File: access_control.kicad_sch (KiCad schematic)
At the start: 64 parts, among them J1 Conn_01x04_Pin, J10 Screw_Terminal_01x02, J2 Screw_Terminal_01x04, J3 Screw_Terminal_01x04, J4 Screw_Terminal_01x02, J5 Screw_Terminal_01x04, J6 Screw_Terminal_01x04, J7 Screw_Terminal_01x02, J8 Screw_Terminal_01x02, J9 Screw_Terminal_01x02, Q1 NMOS, Q2 NMOS, Q3 NMOS, Q4 NMOS, SW1 Reset button, U1 STM32F446RETx, U2 DS3231M, U3 MAX3232ESE, U4 MAX3232ESE, U5 BA033CC0T, Y1 16MHz

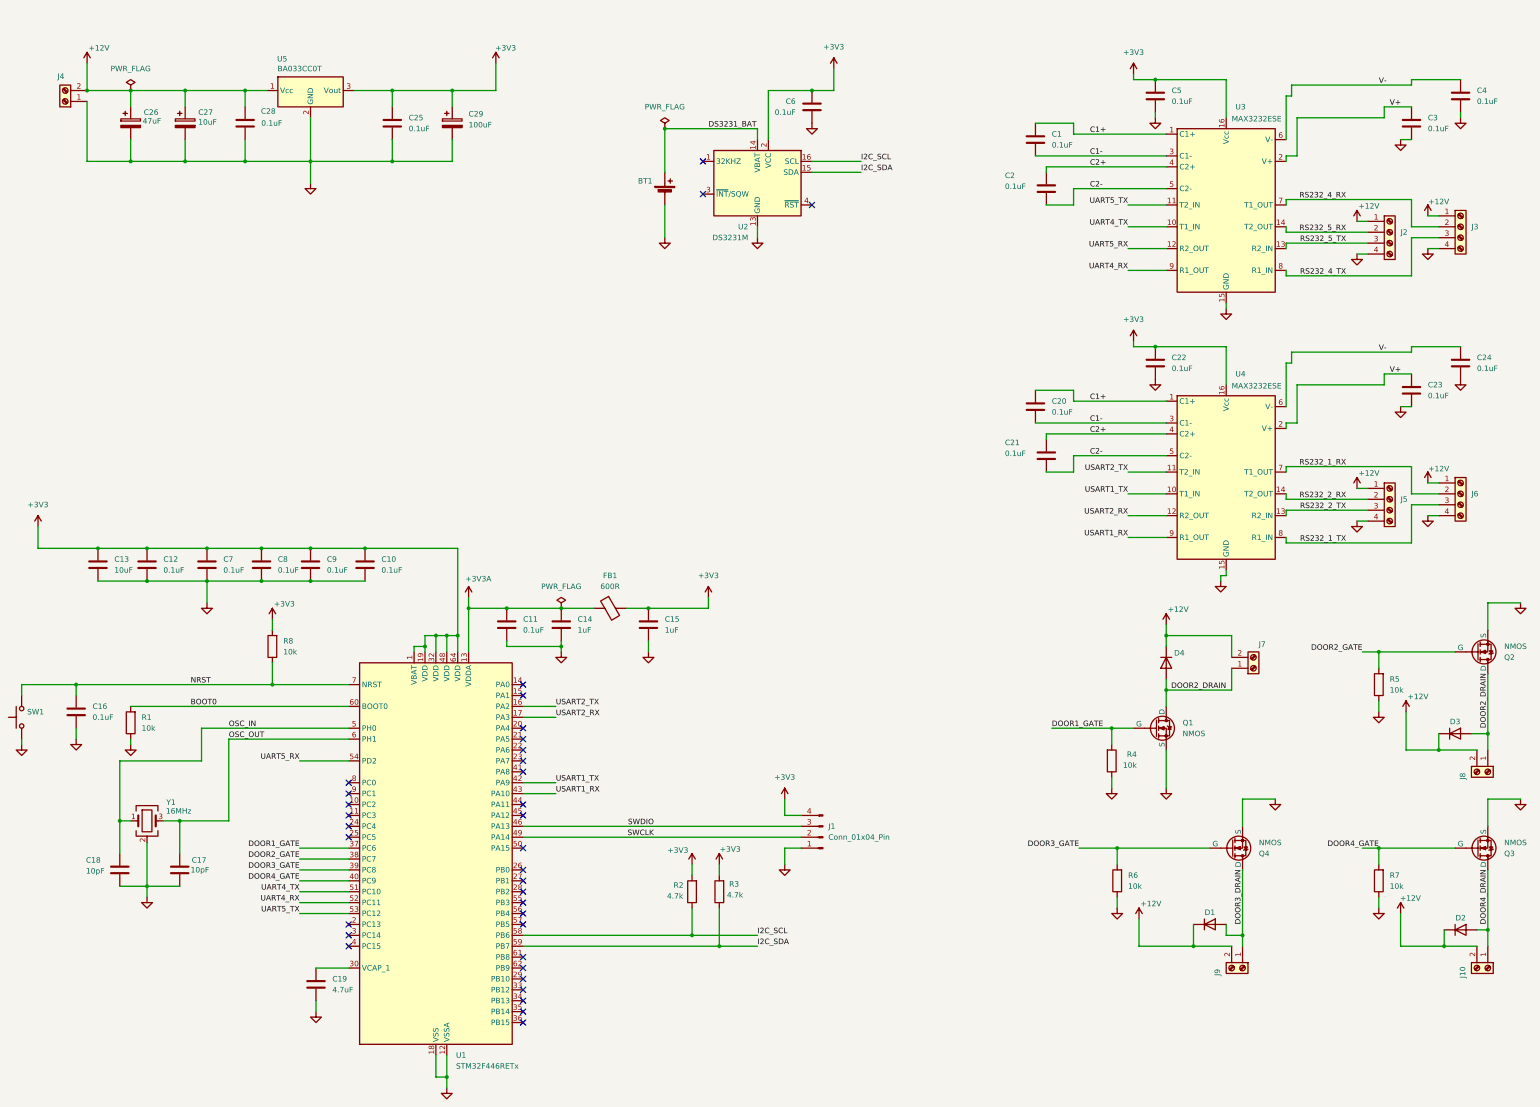
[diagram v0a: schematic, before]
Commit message: ERC check verified
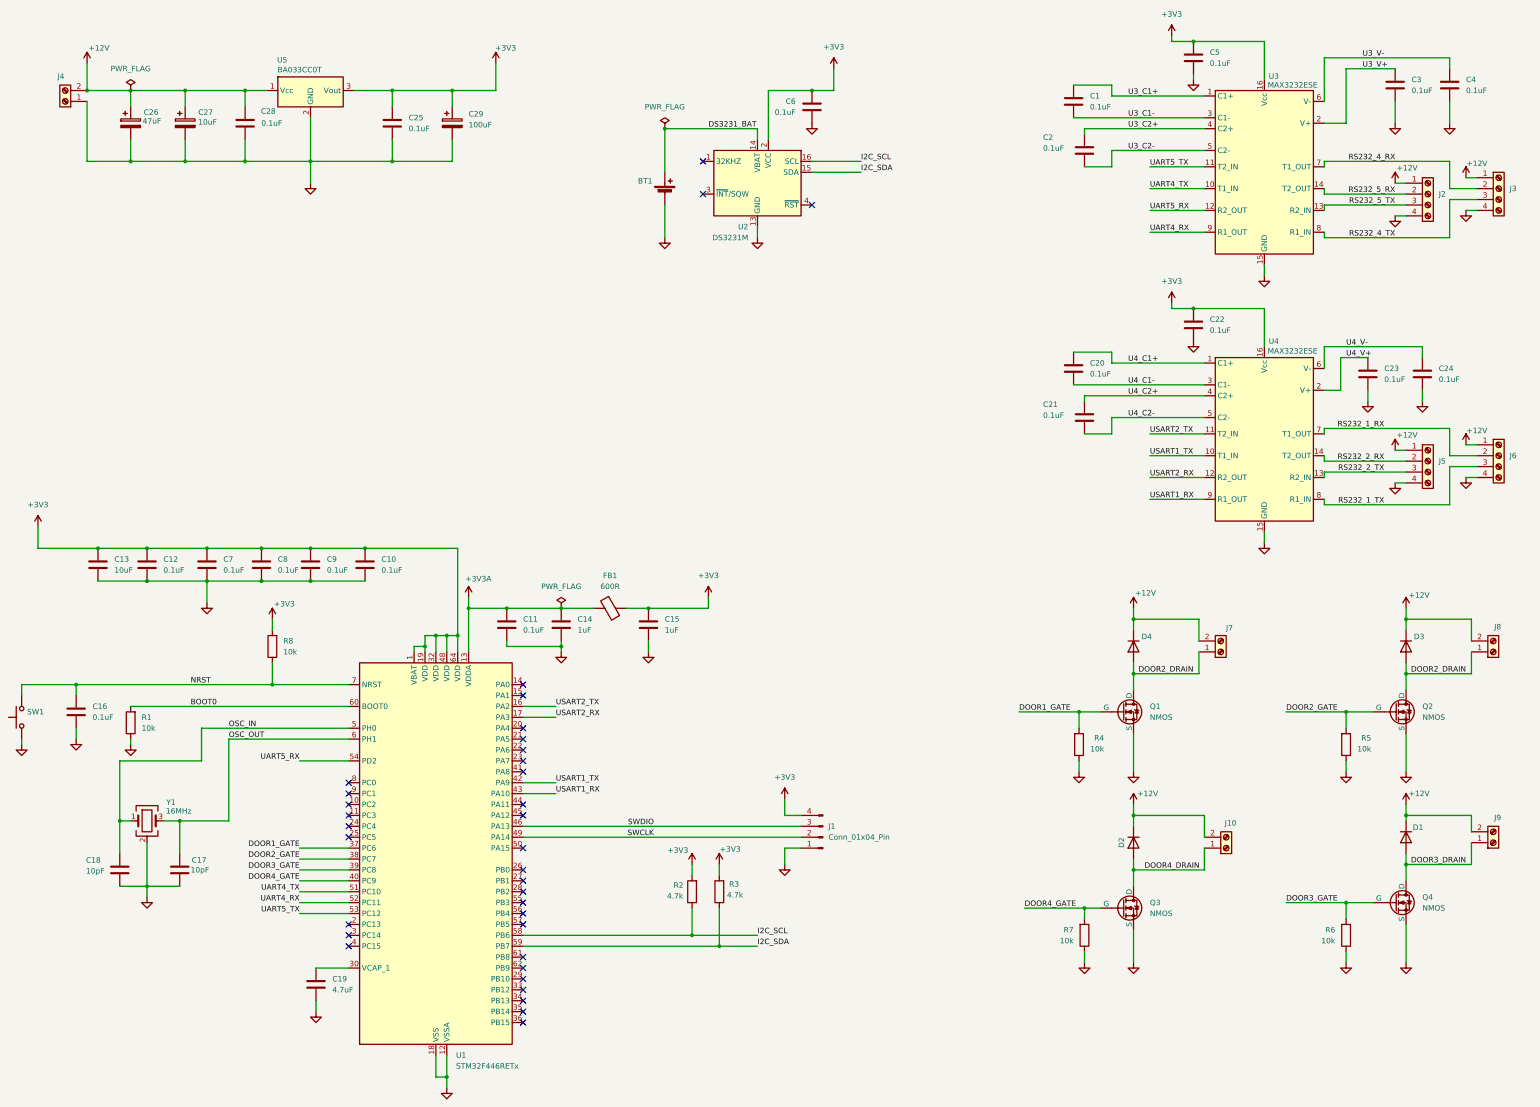
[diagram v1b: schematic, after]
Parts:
- U3, U4: Manufacturer Part Number MAX3232ESE+ -> (none)
- U5: footprint Package_TO_SOT_THT:TO-220-3_Vertical -> (none)
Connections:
- net C1+ renamed U3_C1+
- net U3_C1+: no longer C20.1, U4.1 (C1+)
- net C1- renamed U3_C1-
- net U3_C1-: no longer C20.2, U4.3 (C1-)
- net C2+ renamed U3_C2+
- net U3_C2+: no longer C21.1, U4.4 (C2+)
- net C2- renamed U3_C2-
- net U3_C2-: no longer C21.2, U4.5 (C2-)
- net V+ renamed U3_V+
- net U3_V+: no longer C23.1, U4.2 (V+)
- net V- renamed U3_V-
- net U3_V-: no longer C24.1, U4.6 (V-)
- new net U4_C1+: C20.1, U4.1 (C1+)
- new net U4_C1-: C20.2, U4.3 (C1-)
- new net U4_C2+: C21.1, U4.4 (C2+)
- new net U4_C2-: C21.2, U4.5 (C2-)
- new net U4_V+: C23.1, U4.2 (V+)
- new net U4_V-: C24.1, U4.6 (V-)
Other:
- moved on the sheet: C1, C2, C20, C21, C22, C23, C24, C3, C4, C5, D1, D2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
